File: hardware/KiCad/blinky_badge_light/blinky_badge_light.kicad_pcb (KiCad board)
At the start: 4 copper layers, 135.8 x 109.7 mm, 99 parts, among them Q2 Q_PMOS_GSD, SW1 TS-1187A-B-A-B, U1 ESP32-S3-WROOM-1, U2 TP4056, U3 AP2112K-3.3, U4 MT3608, U5 CP2102N-Axx-xQFN24, U6 SN74LVC1T45DBV

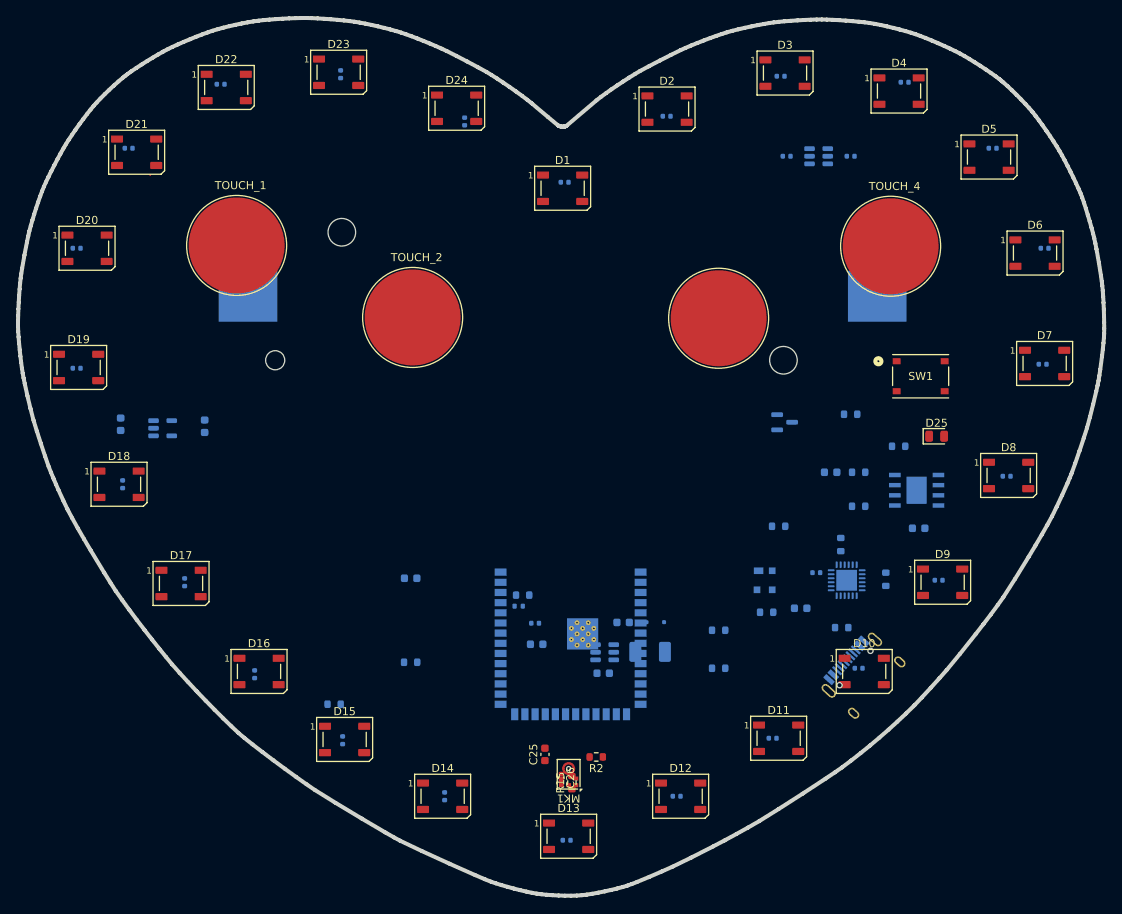
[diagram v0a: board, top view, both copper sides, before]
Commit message: placing items on the board
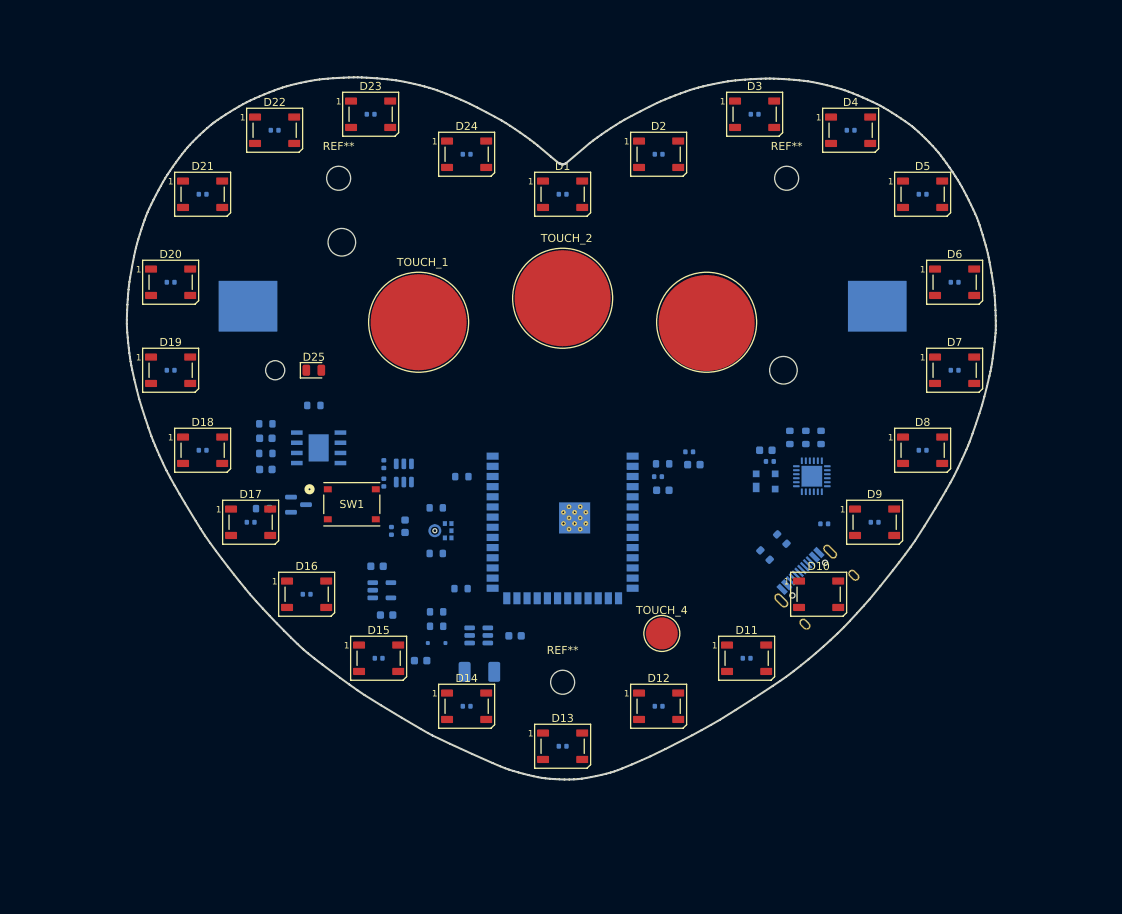
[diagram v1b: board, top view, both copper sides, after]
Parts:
- added REF**: MountingHole_3mm, MountingHole:MountingHole_3mm, F.Cu at (122.0, 65.0)
- added REF**: MountingHole_3mm, MountingHole:MountingHole_3mm, F.Cu at (178.0, 65.0)
- added REF**: MountingHole_3mm, MountingHole:MountingHole_3mm, F.Cu at (150.0, 128.0)
- C25, C26, MK1, R15, R2: moved to B.Cu
- C31: footprint Resistor_SMD:R_0402_1005Metric -> Capacitor_SMD:C_0402_1005Metric
- TOUCH_4: footprint footprints:TestPoint_Pad_D12.0mm -> TestPoint:TestPoint_Pad_D4.0mm
- moved C33 81.9 mm to (112.9, 101.4)
- moved D25 78.3 mm to (118.9, 89.0)
- moved U2 74.9 mm to (119.5, 98.7)
- moved R9 74.4 mm to (112.5, 106.3)
- moved R4 74.4 mm to (112.9, 99.4), turned to 180 degrees
- moved R3 74.3 mm to (112.9, 95.7)
- moved R14 73.3 mm to (118.9, 93.4)
- moved SW1 72.9 mm to (123.6, 105.8)
- moved C32 70.7 mm to (112.9, 97.5), turned to 180 degrees
- moved C37 69.9 mm to (127.7, 100.7), turned to 90 degrees
- moved U6 65.2 mm to (130.2, 101.8), turned to -90 degrees
- moved C36 64.8 mm to (127.7, 103.0), turned to -90 degrees
- moved Q2 61.6 mm to (117.0, 105.8)
- moved TOUCH_4 56.2 mm to (162.4, 121.9)
- moved R15 38.3 mm to (134.2, 106.2), turned to 0 degrees
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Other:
- board size 135.8 x 109.7 mm -> 108.6 x 87.8 mm
